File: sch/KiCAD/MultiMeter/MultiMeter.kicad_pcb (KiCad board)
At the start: 2 copper layers, 35.6 x 52.7 mm, 20 parts, among them J1 Conn_01x02_Male, J2 Conn_01x02_Male, J3 Conn_01x03_Male, J4 Conn_01x03_Male, J5 Conn_01x02_Female, J6 Conn_01x15, J7 Conn_01x15

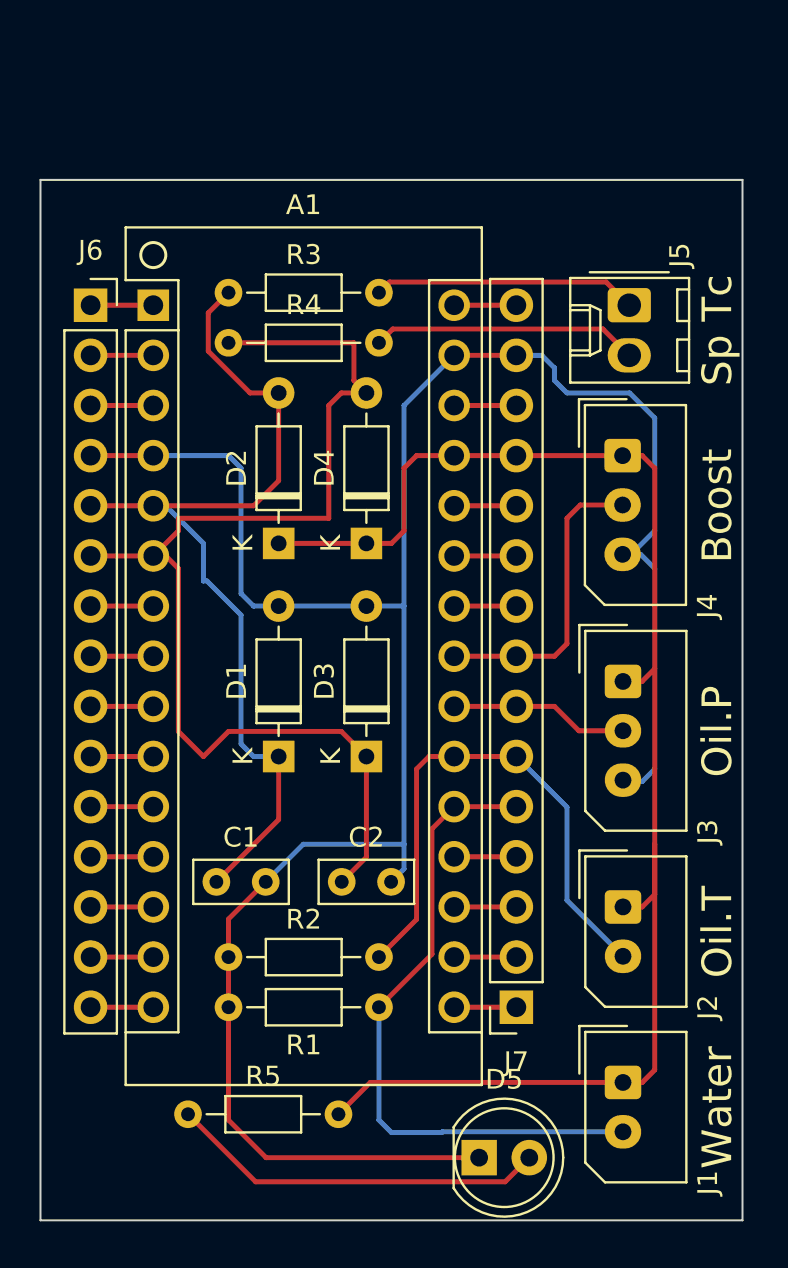
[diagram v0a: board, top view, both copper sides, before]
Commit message: 基板修正
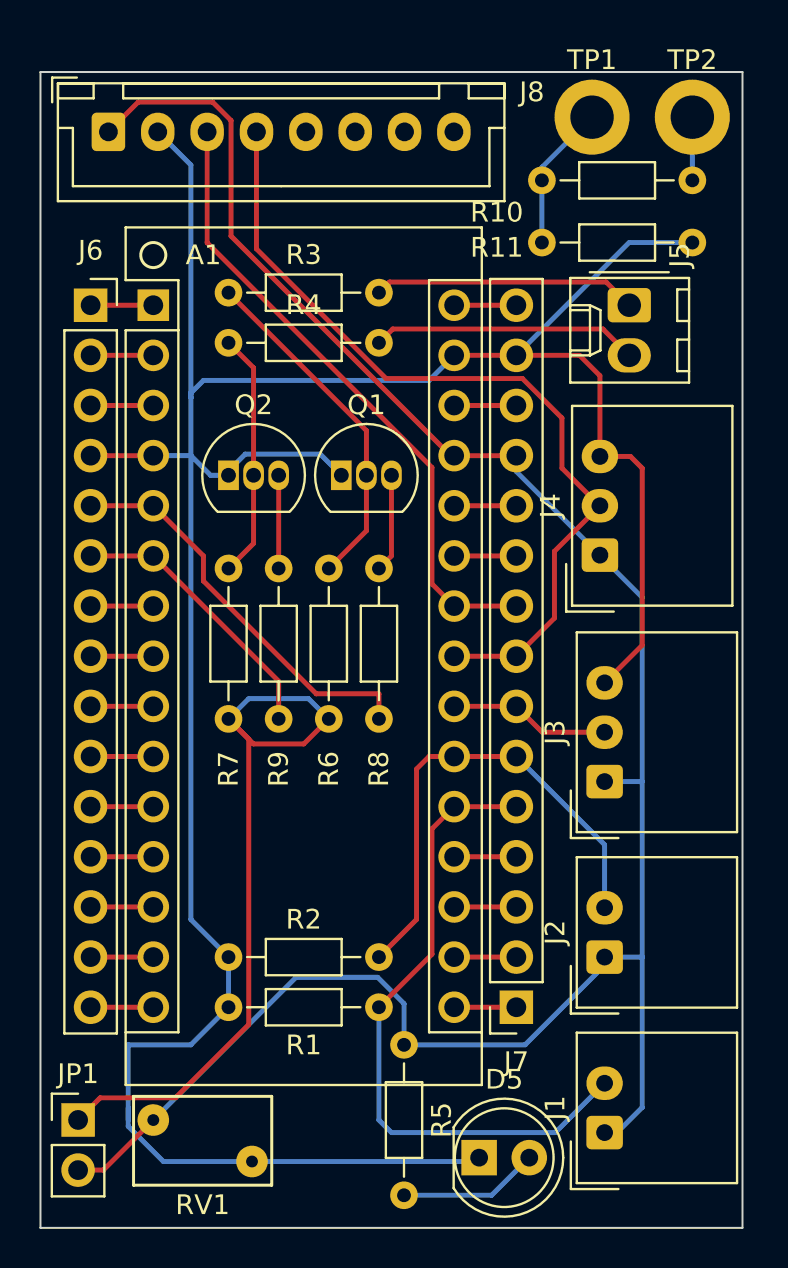
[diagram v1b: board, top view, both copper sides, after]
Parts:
- removed C1, C2: 0.1uF, Capacitor_THT:C_Rect_L4.6mm_W2.0mm_P2.50mm_MKS02_FKP02
- removed D1, D2, D3, D4: 1N4148, Diode_THT:D_DO-35_SOD27_P7.62mm_Horizontal
- added J8: Conn_01x08_Female, Connector_JST:JST_XH_B8B-XH-A_1x08_P2.50mm_Vertical, F.Cu at (40.3, 17.3)
- added JP1: Jumper_2_Open, Connector_PinHeader_2.54mm:PinHeader_1x02_P2.54mm_Vertical, F.Cu at (38.7, 67.3)
- added Q1: 2SC1815, Package_TO_SOT_THT:TO-92_Inline, F.Cu at (52.1, 34.6)
- added Q2: 2SC1815, Package_TO_SOT_THT:TO-92_Inline, F.Cu at (46.4, 34.6)
- added R10: 7K ohm, Resistor_THT:R_Axial_DIN0204_L3.6mm_D1.6mm_P7.62mm_Horizontal, F.Cu at (62.2, 19.7)
- added R11: 5K ohm, Resistor_THT:R_Axial_DIN0204_L3.6mm_D1.6mm_P7.62mm_Horizontal, F.Cu at (62.2, 22.9)
- added R6: 10K ohm, Resistor_THT:R_Axial_DIN0204_L3.6mm_D1.6mm_P7.62mm_Horizontal, F.Cu at (51.4, 39.4)
- added R7: 10K ohm, Resistor_THT:R_Axial_DIN0204_L3.6mm_D1.6mm_P7.62mm_Horizontal, F.Cu at (46.4, 39.4)
- added R8: 10K ohm, Resistor_THT:R_Axial_DIN0204_L3.6mm_D1.6mm_P7.62mm_Horizontal, F.Cu at (54.0, 47.0)
- added R9: 10K ohm, Resistor_THT:R_Axial_DIN0204_L3.6mm_D1.6mm_P7.62mm_Horizontal, F.Cu at (48.9, 47.0)
- added RV1: RV_Disc_D7mm_W4.5mm_P5mm, Varistor:RV_Disc_D7mm_W4.5mm_P5mm, F.Cu at (42.5, 67.3)
- added TP1: TestPoint, MountingHole:MountingHole_2.2mm_M2_DIN965_Pad, F.Cu at (64.8, 16.5)
- added TP2: TestPoint, MountingHole:MountingHole_2.2mm_M2_DIN965_Pad, F.Cu at (69.8, 16.5)
- J1, J2: footprint Connector_Molex:Molex_SPOX_5267-02A_1x02_P2.50mm_Vertical -> Connector_Molex:Molex_SPOX_5268-02A_1x02_P2.50mm_Horizontal
- J3, J4: footprint Connector_Molex:Molex_SPOX_5267-03A_1x03_P2.50mm_Vertical -> Connector_Molex:Molex_SPOX_5268-03A_1x03_P2.50mm_Horizontal
- moved R5 11.7 mm to (55.2, 71.1), turned to 90 degrees
- moved J4 5.17 mm to (65.2, 38.7), turned to 90 degrees
- moved J3 5.16 mm to (65.4, 50.2), turned to 90 degrees
- moved J2 2.71 mm to (65.4, 59.1), turned to 90 degrees
- moved J1 2.71 mm to (65.4, 67.9), turned to 90 degrees
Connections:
- net Net-(A1-Pad27) renamed +5V
- net Net-(A1-Pad29) renamed GNDPWR
- R3 pad 1: Net-(A1-Pad5) -> Net-(Q1-Pad2)
- R4 pad 1: Net-(A1-Pad6) -> Net-(Q2-Pad2)
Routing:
- net Net-(A1-Pad6): track 57.4 -> 14.1 mm
- net Net-(JP1-Pad1): track 0.00 -> 38.6 mm
- net +5V: track 76.7 -> 109.5 mm
- net Net-(A1-Pad24): track 3.15 -> 32.4 mm
- net Net-(A1-Pad23): track 15.4 -> 42.7 mm
- net Net-(A1-Pad5): track 45.9 -> 20.6 mm
- net GNDPWR: track 118.4 -> 140.5 mm
- net Net-(Q1-Pad2): track 0.00 -> 17.7 mm
- net Net-(Q2-Pad2): track 0.00 -> 12.5 mm
- net Net-(D5-Pad2): track 19.2 -> 7.13 mm
- net Net-(R10-Pad1): track 0.00 -> 7.40 mm
- net Net-(Q1-Pad3): track 0.00 -> 4.98 mm
- net Net-(Q2-Pad3): track 0.00 -> 4.72 mm
- net throttle(+12V - 0V): track 0.00 -> 3.20 mm
- net Net-(A1-Pad21): track 28.0 -> 25.1 mm
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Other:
- board size 35.6 x 52.7 mm -> 35.6 x 58.5 mm
- board text added: "2023/07/01"
- board text removed: "2022/09/13"
